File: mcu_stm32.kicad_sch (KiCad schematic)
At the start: 20 parts, among them J1 Debug, J2 Boot_Sel, SW1 RESET, U1 STM32F103C8Tx, Y1 8mHz

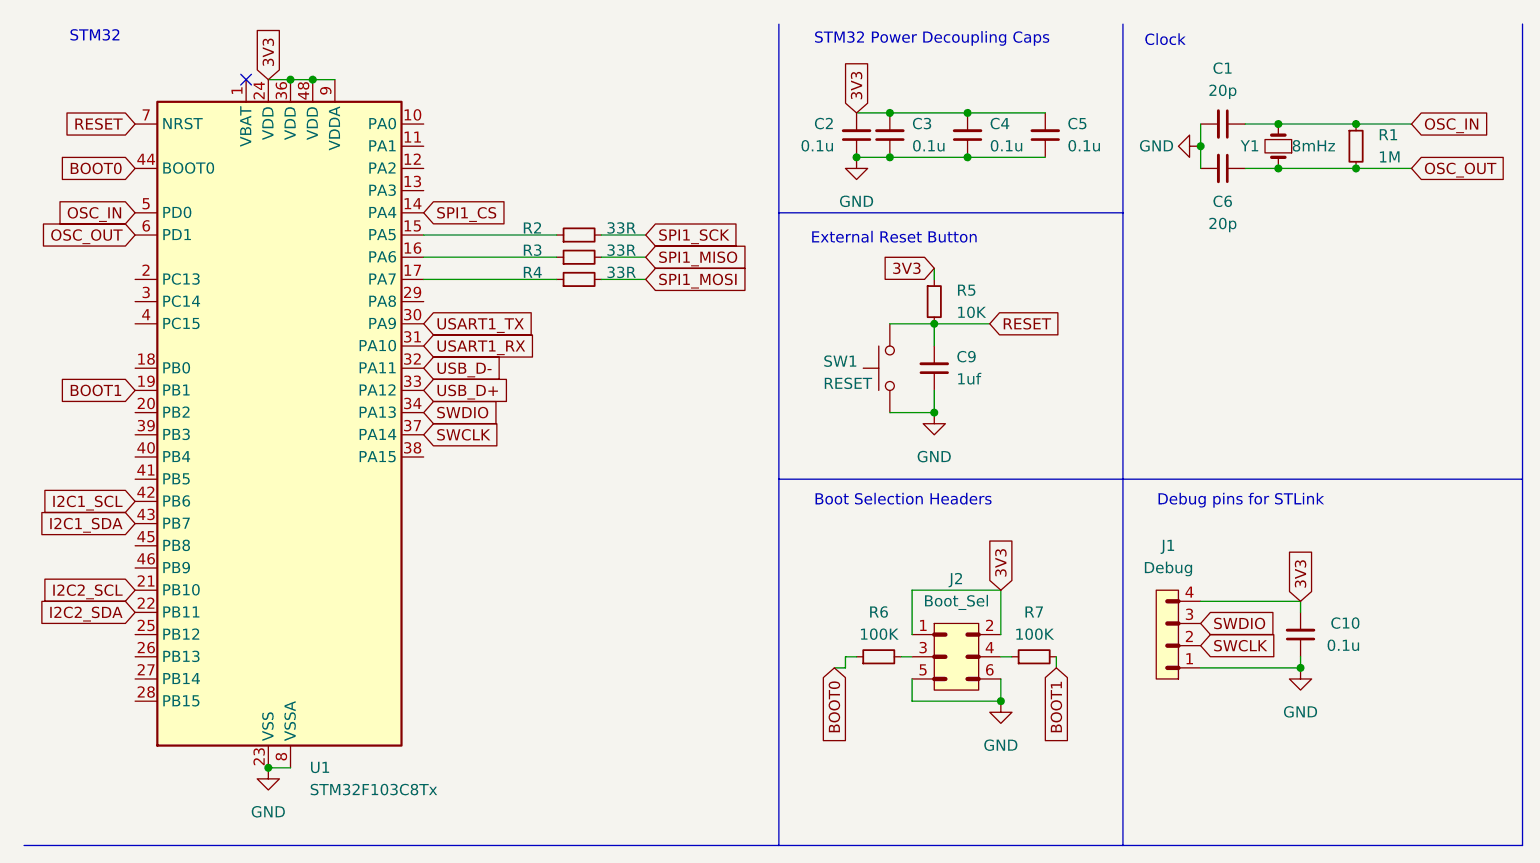
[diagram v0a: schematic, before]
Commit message: esp32 silindi, yerleştirmeler yapıldı
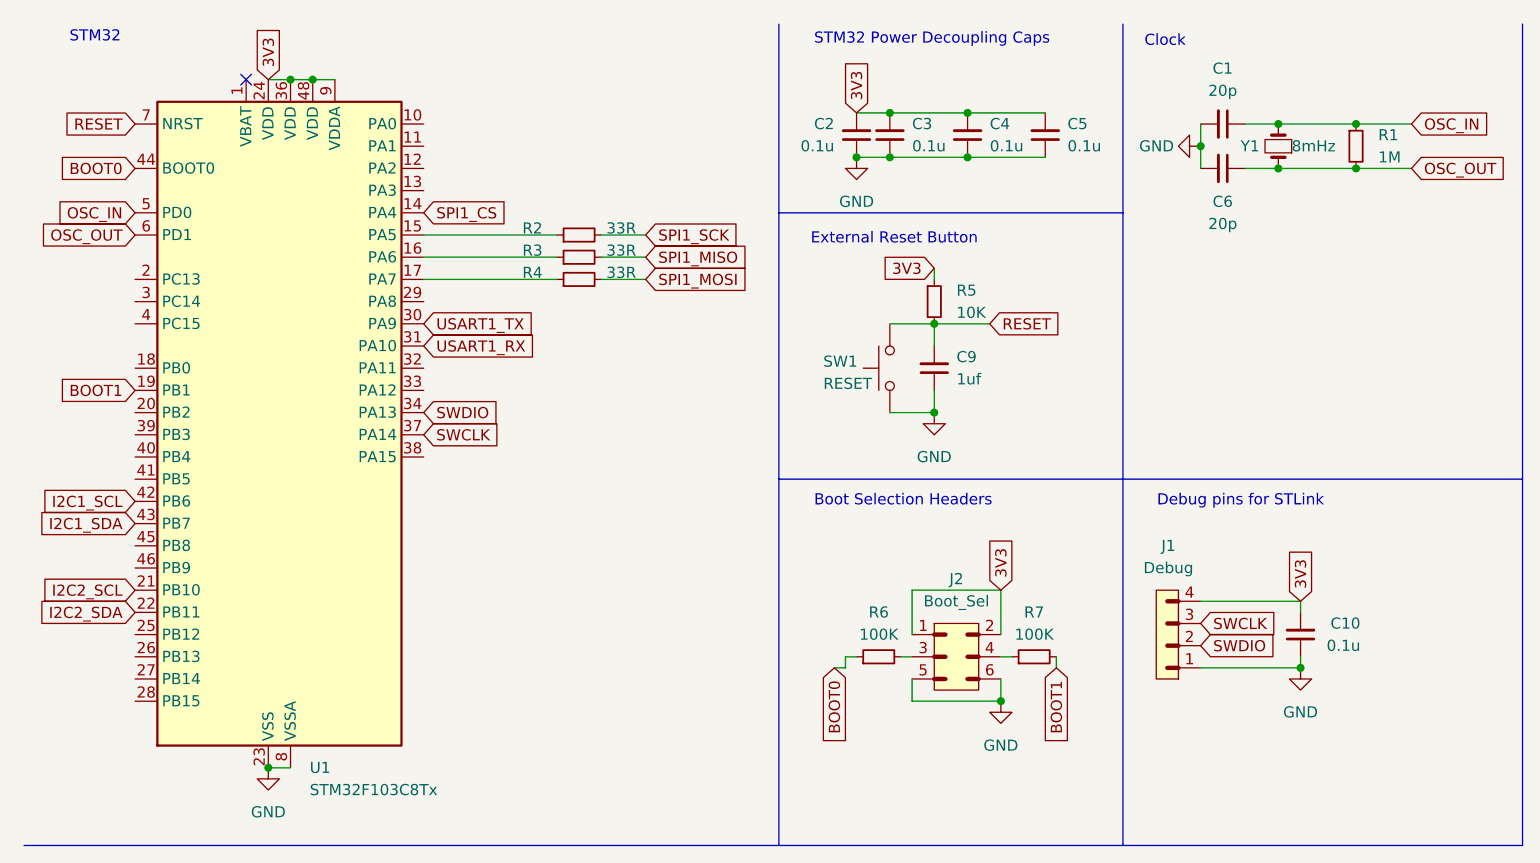
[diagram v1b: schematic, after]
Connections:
- net SWCLK: now also J1.3; no longer J1.2
- net SWDIO: now also J1.2; no longer J1.3
- net USB_D+: no longer names the net of U1.33 (PA12)
- net USB_D-: no longer names the net of U1.32 (PA11)
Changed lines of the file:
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@@
-		)
-	)
-	(global_label "USB_D+"
-		(shape input)
-		(at 58.42 55.88 0)
-		(fields_autoplaced yes)
-		(effects
-			(font
-				(size 1.27 1.27)
-			)
-			(justify left)
-		)
-		(property "Intersheetrefs" "${INTERSHEET_REFS}"
-			(at 69.0252 55.88 0)
-			(effects
-				(font
-					(size 1.27 1.27)
-				)
-				(justify left)
-				(hide yes)
-			)
 		)
 	)
@@
 	(global_label "SWCLK"
 		(shape input)
+		(at 147.32 82.55 0)
+		(fields_autoplaced yes)
+		(effects
+			(font
+				(size 1.27 1.27)
+			)
+			(justify left)
+		)
+		(property "Intersheetrefs" "${INTERSHEET_REFS}"
+			(at 156.5342 82.55 0)
+			(effects
+				(font
+					(size 1.27 1.27)
+				)
+				(justify left)
+				(hide yes)
+			)
+		)
+	)
+	(global_label "OSC_IN"
+		(shape input)
+		(at 25.4 35.56 180)
+		(fields_autoplaced yes)
+		(effects
+			(font
+				(size 1.27 1.27)
+			)
+			(justify right)
+		)
+		(property "Intersheetrefs" "${INTERSHEET_REFS}"
+			(at 15.7019 35.56 0)
+			(effects
+				(font
+					(size 1.27 1.27)
+				)
+				(justify right)
+				(hide yes)
+			)
+		)
+	)
+	(global_label "3V3"
+		(shape input)
+		(at 116.84 41.91 180)
+		(fields_autoplaced yes)
+		(effects
+			(font
+				(size 1.27 1.27)
+			)
+			(justify right)
+		)
+		(property "Intersheetrefs" "${INTERSHEET_REFS}"
+			(at 110.3472 41.91 0)
+			(effects
+				(font
+					(size 1.27 1.27)
+				)
+				(justify right)
+				(hide yes)
+			)
+		)
+	)
+	(global_label "3V3"
+		(shape input)
+		(at 124.46 78.74 90)
+		(fields_autoplaced yes)
+		(effects
+			(font
+				(size 1.27 1.27)
+			)
+			(justify left)
+		)
+		(property "Intersheetrefs" "${INTERSHEET_REFS}"
+			(at 124.46 72.2472 90)
+			(effects
+				(font
+					(size 1.27 1.27)
+				)
+				(justify left)
+				(hide yes)
+			)
+		)
+	)
+	(global_label "SWDIO"
+		(shape input)
 		(at 147.32 85.09 0)
 		(fields_autoplaced yes)
@@
 		)
 		(property "Intersheetrefs" "${INTERSHEET_REFS}"
-			(at 156.5342 85.09 0)
-			(effects
-				(font
-					(size 1.27 1.27)
-				)
-				(justify left)
-				(hide yes)
-			)
-		)
-	)
-	(global_label "OSC_IN"
-		(shape input)
-		(at 25.4 35.56 180)
-		(fields_autoplaced yes)
-		(effects
-			(font
-				(size 1.27 1.27)
-			)
-			(justify right)
-		)
-		(property "Intersheetrefs" "${INTERSHEET_REFS}"
-			(at 15.7019 35.56 0)
-			(effects
-				(font
-					(size 1.27 1.27)
-				)
-				(justify right)
-				(hide yes)
-			)
-		)
-	)
-	(global_label "3V3"
-		(shape input)
-		(at 116.84 41.91 180)
-		(fields_autoplaced yes)
-		(effects
-			(font
-				(size 1.27 1.27)
-			)
-			(justify right)
-		)
-		(property "Intersheetrefs" "${INTERSHEET_REFS}"
-			(at 110.3472 41.91 0)
-			(effects
-				(font
-					(size 1.27 1.27)
-				)
-				(justify right)
-				(hide yes)
-			)
-		)
-	)
-	(global_label "USB_D-"
-		(shape input)
-		(at 58.42 53.34 0)
-		(fields_autoplaced yes)
-		(effects
-			(font
-				(size 1.27 1.27)
-			)
-			(justify left)
-		)
-		(property "Intersheetrefs" "${INTERSHEET_REFS}"
-			(at 69.0252 53.34 0)
-			(effects
-				(font
-					(size 1.27 1.27)
-				)
-				(justify left)
-				(hide yes)
-			)
-		)
-	)
-	(global_label "3V3"
-		(shape input)
-		(at 124.46 78.74 90)
-		(fields_autoplaced yes)
-		(effects
-			(font
-				(size 1.27 1.27)
-			)
-			(justify left)
-		)
-		(property "Intersheetrefs" "${INTERSHEET_REFS}"
-			(at 124.46 72.2472 90)
-			(effects
-				(font
-					(size 1.27 1.27)
-				)
-				(justify left)
-				(hide yes)
-			)
-		)
-	)
-	(global_label "SWDIO"
-		(shape input)
-		(at 147.32 82.55 0)
-		(fields_autoplaced yes)
-		(effects
-			(font
-				(size 1.27 1.27)
-			)
-			(justify left)
-		)
-		(property "Intersheetrefs" "${INTERSHEET_REFS}"
-			(at 156.1714 82.55 0)
-			(effects
-				(font
+			(at 156.1714 85.09 0)
+			(effects
+				(font

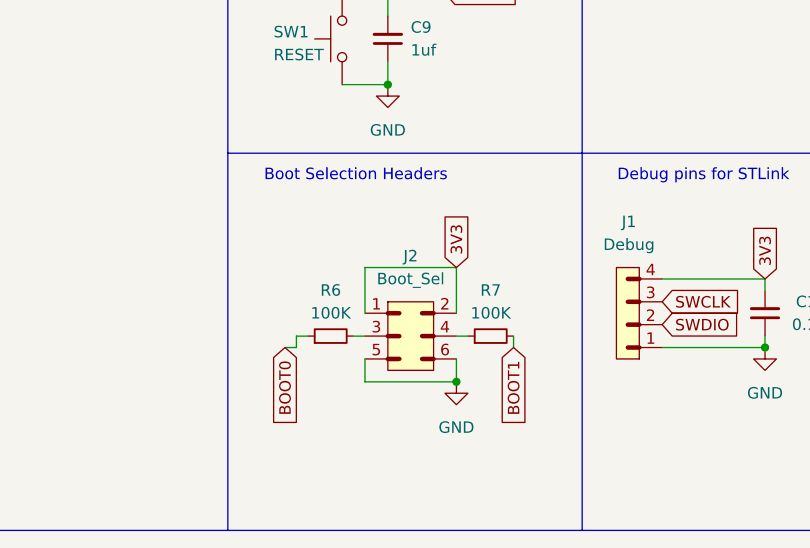
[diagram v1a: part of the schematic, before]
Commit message: Routing
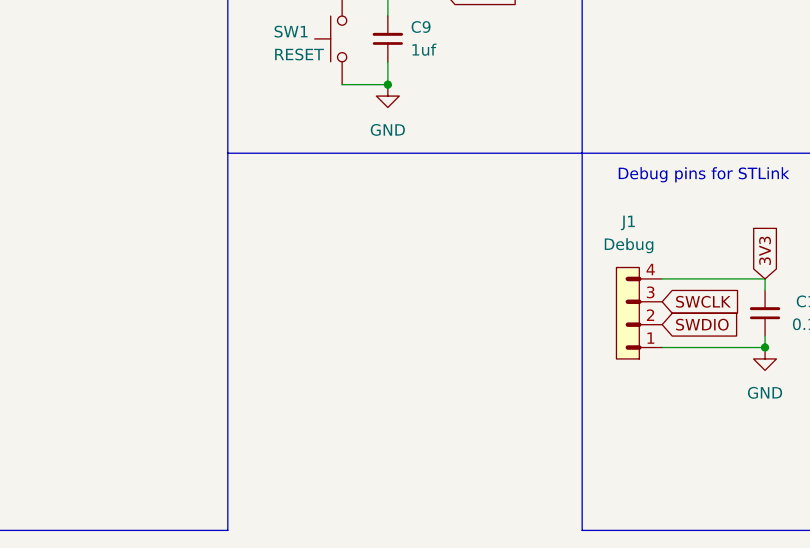
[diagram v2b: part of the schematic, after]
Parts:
- removed J2: Boot_Sel, Connector_PinHeader_2.54mm:PinHeader_2x03_P2.54mm_Vertical, symbol PCM_SL_Pin_Headers:PINHD_2x3_Male
- removed R6, R7: 100K, Resistor_SMD:R_0805_2012Metric, symbol Device:R_Small
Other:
- note removed: "Boot Selection Headers"
